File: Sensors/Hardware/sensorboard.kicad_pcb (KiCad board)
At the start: 4 copper layers, 100 x 50 mm, 298 parts, among them J1 RBUS, J10 1053131104, J11 1053131104, J12 1053131104, J13 1053131104, J14 1053131104, J15 USB_C_Receptacle_USB2.0, J16 Micro_SD_Card_Det, J2 Conn_Coaxial, J3 1053131104, J4 1053131104, J5 1053131104, J6 1053131104, J7 1053131104, J8 1053131104, J9 1053131104, U1 ESP32-S3, U10 ADS131M06IRSNR, U11 TPS61092RSAR, U12 LM2623QNHLRQ1, U13 SN65HVD230, U2 MAX31856, U3 MAX31856, U4 MAX31856, U5 MAX31856, U6 LM66200DRLR, U7 MAX77827AEFD+T, U8 SC4215, U9 ADS131M06IRSNR, Y1 40MHz±10ppm

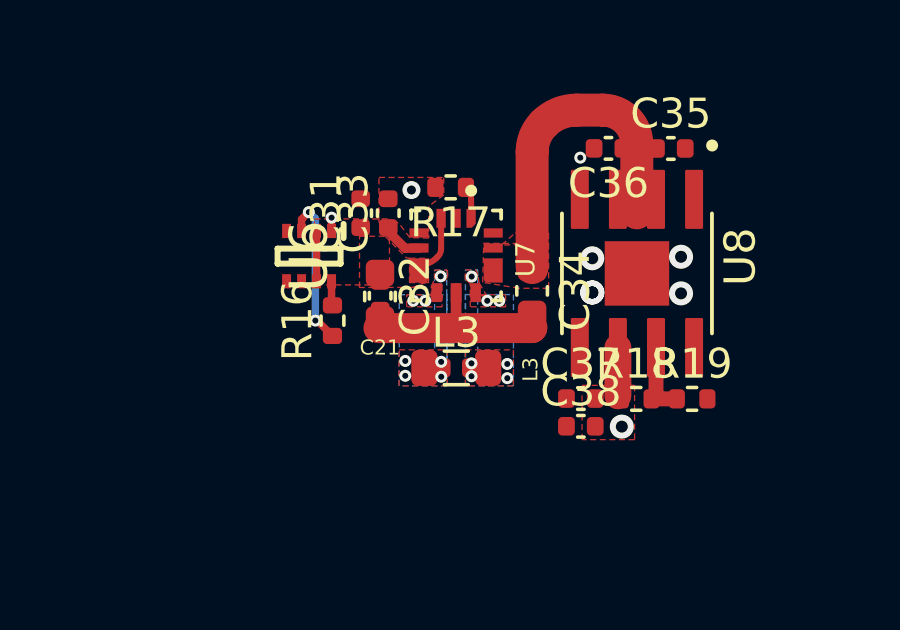
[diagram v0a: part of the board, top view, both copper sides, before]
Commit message: power layout done
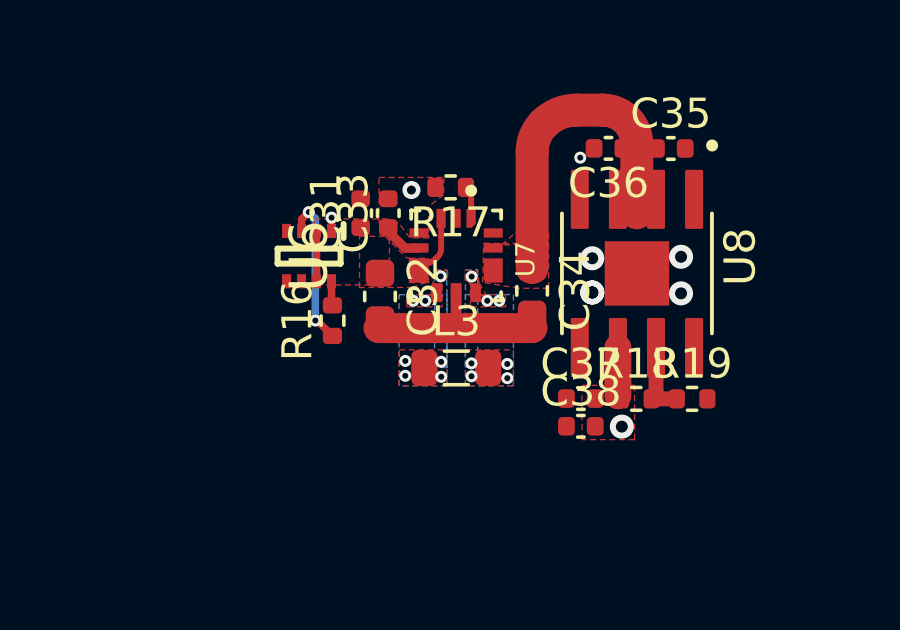
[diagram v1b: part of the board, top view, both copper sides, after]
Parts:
- removed the C21 at (123.4, 134.9)
- removed the L3 at (125.9, 137.3)
- C32: footprint Capacitor_SMD:C_0402_1005Metric -> Capacitor_SMD:C_0603_1608Metric
- L3: footprint Inductor_SMD:L_0402_1005Metric -> Inductor_SMD:L_0805_2012Metric
